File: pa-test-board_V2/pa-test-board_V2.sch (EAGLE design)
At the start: 34 parts, among them J1 142-0701-851, J2 142-0701-851, J3 142-0701-851, J4 142-0701-851, SW1 TL36PO, U10 TQP9111

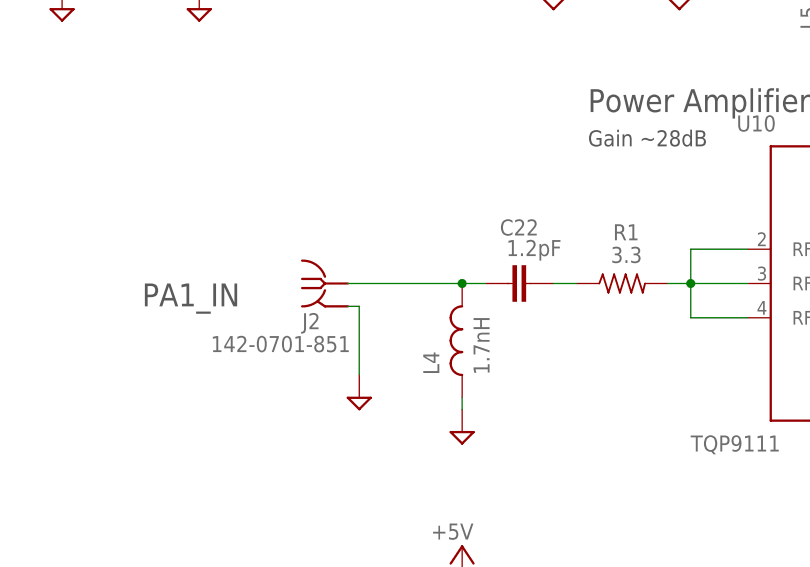
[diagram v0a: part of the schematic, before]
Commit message: Added 1st draft layout for Oliver
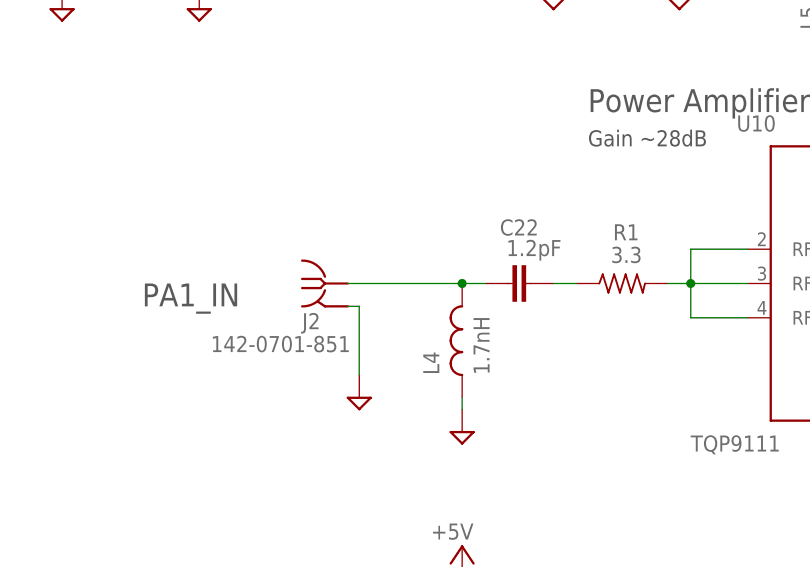
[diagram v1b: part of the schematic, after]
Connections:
- removed net N$25: C22.1, L4.2
- net N$1: now also C22.1, L4.2
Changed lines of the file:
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@@
 <?xml version="1.0" encoding="utf-8"?>
 <!DOCTYPE eagle SYSTEM "eagle.dtd">
-<eagle version="9.5.1">
+<eagle version="9.6.1">
 <drawing>
 <settings>
@@
 <setting verticaltext="up"/>
 </settings>
-<grid distance="0.05" unitdist="inch" unit="inch" style="lines" multiple="2" display="yes" altdistance="0.01" altunitdist="inch" altunit="inch"/>
+<grid distance="0.1" unitdist="inch" unit="inch" style="lines" multiple="1" display="no" altdistance="0.01" altunitdist="inch" altunit="inch"/>
 <layers>
 <layer number="1" name="Top" color="4" fill="1" visible="no" active="no"/>
@@
 </segment>
 </net>
-<net name="N$25" class="1">
-<segment>
-<pinref part="C22" gate="CE" pin="1"/>
-<wire x1="86.36" y1="119.38" x2="83.82" y2="119.38" width="0.1524" layer="91"/>
-<pinref part="L4" gate="L" pin="2"/>
-<wire x1="83.82" y1="119.38" x2="76.2" y2="119.38" width="0.1524" layer="91"/>
-<junction x="83.82" y="119.38"/>
-</segment>
-</net>
 <net name="N$27" class="1">
 <segment>
@@
 <segment>
 <pinref part="J2" gate="G$1" pin="RF"/>
-<wire x1="71.12" y1="119.38" x2="76.2" y2="119.38" width="0.1524" layer="91"/>
-</segment>
-</net>
+<pinref part="C22" gate="CE" pin="1"/>
+<wire x1="86.36" y1="119.38" x2="83.82" y2="119.38" width="0.1524" layer="91"/>
+<pinref part="L4" gate="L" pin="2"/>
+<wire x1="83.82" y1="119.38" x2="71.12" y2="119.38" width="0.1524" layer="91"/>
+<junction x="83.82" y="119.38"/>
+</segment>
+</net>
